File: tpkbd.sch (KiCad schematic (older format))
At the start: 21 parts, among them CON1 AVR-ISP-6, J1 CONN_01X02, J2 CONN_01X01, J3 USB_OTG, J4 CONN_02X20, J5 CONN_01X04, J6 GS2, J7 0, U1 ATMEGA8515-16AU, U2 AP111733, Y1 Crystal_GND24

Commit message: cleanup
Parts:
- removed CON1: AVR-ISP-6, Pin_Headers:Pin_Header_Straight_2x03, symbol AVR-ISP-6
- added D1: LED, KX14:PLCC4, symbol LED_Dual_AACC
- added J?: CONN_02X10, symbol CONN_02X10
- added R6, R7, R8: R, Resistors_SMD:R_0603_HandSoldering, symbol R
- C1, C2: footprint Capacitors_SMD:C_0805_HandSoldering -> Capacitors_SMD:C_0603_HandSoldering
- C3: footprint Capacitors_SMD:C_0402 -> Capacitors_SMD:C_0603_HandSoldering
- J2: footprint Pin_Headers:Pin_Header_Straight_1x01 -> KX14:Pins1x1
- J4: value CONN_02X20 -> CONN_02X21; symbol CONN_02X20 -> CONN_02X21
- R1, R2, R3, R4, R5: footprint Resistors_SMD:R_0805_HandSoldering -> Resistors_SMD:R_0603_HandSoldering
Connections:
- net +3V3: now also J?.2 (P2), R6.1; no longer J5.1 (P1)
- net +5V: now also J5.1 (P1)
- net B5: now also J?.4 (P4)
- net B6: now also J?.6 (P6)
- net B7: now also J?.8 (P8)
- net GND: now also J4.41 (P41), J?.12 (P12), R8.2
- net RST: now also J?.10 (P10)
- net kb_id0: now also R7.1; no longer U1.10 ((XCK)PD4)
- net at R3.2: now also U1.10 ((XCK)PD4); no longer U1.9 ((INT1)PD3)
- new net: D1.2 (A2), R6.2
- new net: D1.3 (K1), R8.1
- new net led: D1.1 (A1), D1.4 (K2), R7.2, U1.9 ((INT1)PD3)
- no-connect marks 4 -> 19
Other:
- moved on the sheet: J7, R3

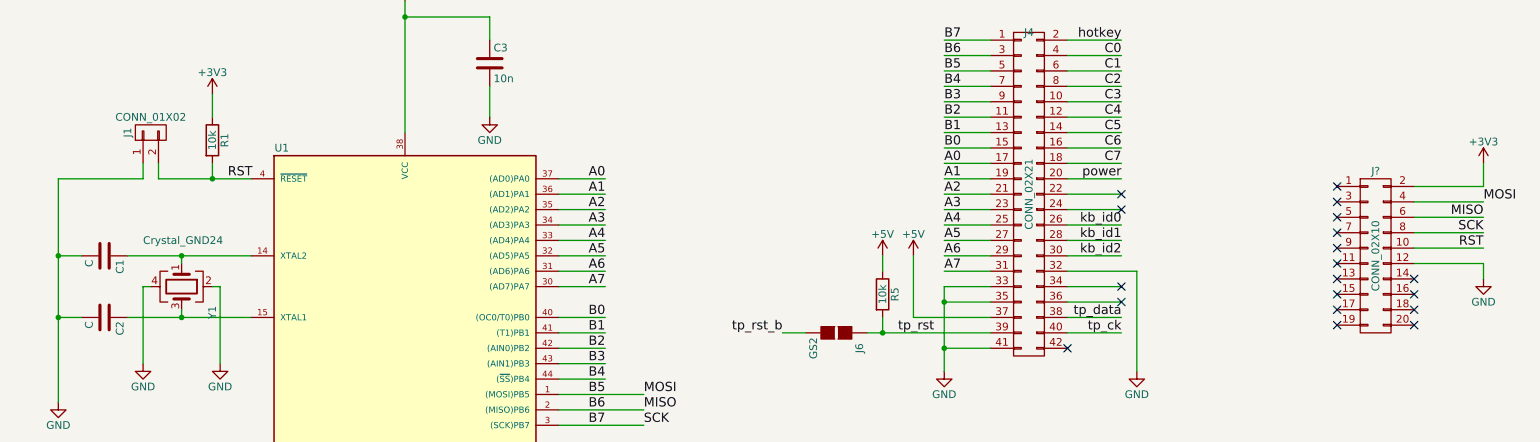
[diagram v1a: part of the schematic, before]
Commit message: cleanup2
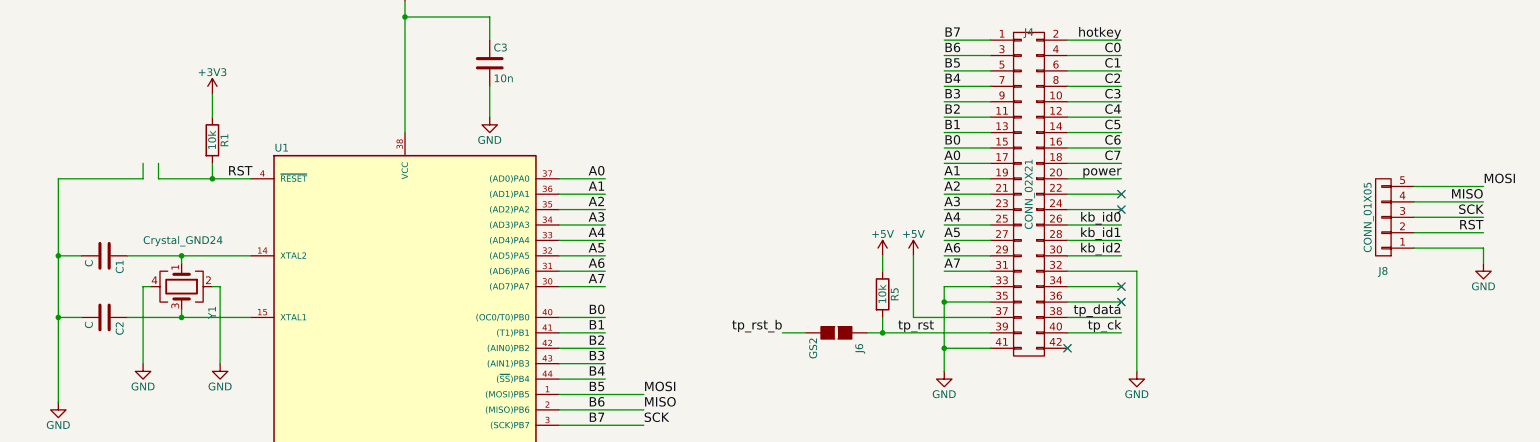
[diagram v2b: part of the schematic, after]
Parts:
- removed J1: CONN_01X02, Buttons_Switches_SMD:SW_SPST_FSMSM, symbol CONN_01X02
- removed J?: CONN_02X10, symbol CONN_02X10
- added J8: CONN_01X05, KX14:Pins_1x5, symbol CONN_01X05
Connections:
- net B5: now also J8.5 (P5)
- net B6: now also J8.4 (P4)
- net B7: now also J8.3 (P3)
- net GND: now also J8.1 (P1)
- net RST: now also J8.2 (P2)
- no-connect marks 19 -> 5
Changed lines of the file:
@@
-$EndComp
-$Comp
-L CONN_01X02 J1
-U 1 1 59BAB43F
-P 1900 2300
-F 0 "J1" H 1900 2450 50  0000 C CNN
-F 1 "CONN_01X02" V 2000 2300 50  0000 C CNN
-F 2 "Buttons_Switches_SMD:SW_SPST_FSMSM" H 1900 2300 50  0001 C CNN
-F 3 "" H 1900 2300 50  0001 C CNN
-	1    1900 2300
-	0    -1   -1   0
 $EndComp
 $Comp
@@
 Text Label 2400 2600 0    60   ~ 0
 RST
-Text Label 10550 3050 2    60   ~ 0
+Text Label 10550 2950 2    60   ~ 0
 RST
 Text Label 7050 2500 0    60   ~ 0
@@
 Connection ~ 6150 5000
 Wire Wire Line
-	10550 3050 10100 3050
+	10550 2950 10100 2950
+Wire Wire Line
+	10550 2750 10100 2750
 Wire Wire Line
 	10550 2850 10100 2850
 Wire Wire Line
-	10550 2950 10100 2950
-Wire Wire Line
 	10100 2650 10550 2650
 Wire Wire Line
-	10100 2750 10550 2750
-Wire Wire Line
-	10100 3150 10550 3150
+	10100 3050 10550 3050
 Wire Wire Line
 	7350 2500 7050 2500
@@
 Wire Wire Line
 	4550 5100 4900 5100
+Text Label 10550 2750 2    60   ~ 0
+MISO
 Text Label 10550 2850 2    60   ~ 0
-MISO
-Text Label 10550 2950 2    60   ~ 0
 SCK
-Text Label 10550 2750 0    60   ~ 0
+Text Label 10550 2650 0    60   ~ 0
 MOSI
 $Comp
 L GND #PWR014
 U 1 1 59BAD155
-P 10550 3250
-F 0 "#PWR014" H 10550 3000 50  0001 C CNN
-F 1 "GND" H 10550 3100 50  0000 C CNN
-F 2 "" H 10550 3250 50  0001 C CNN
-F 3 "" H 10550 3250 50  0001 C CNN
-	1    10550 3250
-	1    0    0    -1
-$EndComp
-Wire Wire Line
-	10550 3150 10550 3250
+P 10550 3150
+F 0 "#PWR014" H 10550 2900 50  0001 C CNN
+F 1 "GND" H 10550 3000 50  0000 C CNN
+F 2 "" H 10550 3150 50  0001 C CNN
+F 3 "" H 10550 3150 50  0001 C CNN
+	1    10550 3150
+	1    0    0    -1
+$EndComp
+Wire Wire Line
+	10550 3050 10550 3150
 Text Label 5100 4100 0    60   ~ 0
 MISO
@@
 	6900 4850 6900 5000
 Connection ~ 6900 5000
-$Comp
-L +3V3 #PWR017
-U 1 1 59BADCC0
-P 10550 2500
-F 0 "#PWR017" H 10550 2350 50  0001 C CNN
-F 1 "+3V3" H 10550 2640 50  0000 C CNN
-F 2 "" H 10550 2500 50  0001 C CNN
-F 3 "" H 10550 2500 50  0001 C CNN
-	1    10550 2500
-	1    0    0    -1
-$EndComp
-Wire Wire Line
-	10550 2650 10550 2500
 Wire Wire Line
 	4100 2200 4100 2000
@@
 	5350 5400 5350 5100
 $Comp
-L GND #PWR018
+L GND #PWR017
 U 1 1 59BAE839
 P 5450 6100
-F 0 "#PWR018" H 5450 5850 50  0001 C CNN
+F 0 "#PWR017" H 5450 5850 50  0001 C CNN
 F 1 "GND" H 5450 5950 50  0000 C CNN
 F 2 "" H 5450 6100 50  0001 C CNN
@@
 	5050 5100 5150 5100
 $Comp
-L PWR_FLAG #FLG019
+L PWR_FLAG #FLG018
 U 1 1 59BAEACE
 P 9100 5450
-F 0 "#FLG019" H 9100 5525 50  0001 C CNN
+F 0 "#FLG018" H 9100 5525 50  0001 C CNN
 F 1 "PWR_FLAG" H 9100 5600 50  0000 C CNN
 F 2 "" H 9100 5450 50  0001 C CNN
@@
 Connection ~ 8500 5600
 $Comp
-L PWR_FLAG #FLG020
+L PWR_FLAG #FLG019
 U 1 1 59BAEC2F
 P 9450 4900
-F 0 "#FLG020" H 9450 4975 50  0001 C CNN
+F 0 "#FLG019" H 9450 4975 50  0001 C CNN
 F 1 "PWR_FLAG" H 9450 5050 50  0000 C CNN
 F 2 "" H 9450 4900 50  0001 C CNN
@@
 $EndComp
 $Comp
-L GND #PWR021
+L GND #PWR020
 U 1 1 59BAF57F
 P 1850 3800
-F 0 "#PWR021" H 1850 3550 50  0001 C CNN
+F 0 "#PWR020" H 1850 3550 50  0001 C CNN
 F 1 "GND" H 1850 3650 50  0000 C CNN
 F 2 "" H 1850 3800 50  0001 C CNN
@@
 	1850 3300 1900 3300
 $Comp
-L GND #PWR022
+L GND #PWR021
 U 1 1 59BAF671
 P 2350 3800
-F 0 "#PWR022" H 2350 3550 50  0001 C CNN
+F 0 "#PWR021" H 2350 3550 50  0001 C CNN
 F 1 "GND" H 2350 3650 50  0000 C CNN
 F 2 "" H 2350 3800 50  0001 C CNN
@@
 	750  6250 750  6350
 $Comp
-L GND #PWR023
+L GND #PWR022
 U 1 1 59BB2E4B
 P 1350 7350
-F 0 "#PWR023" H 1350 7100 50  0001 C CNN
+F 0 "#PWR022" H 1350 7100 50  0001 C CNN
 F 1 "GND" H 1350 7200 50  0000 C CNN
 F 2 "" H 1350 7350 50  0001 C CNN
@@
 	1350 6950 1350 7350
 $Comp
-L PWR_FLAG #FLG024
+L PWR_FLAG #FLG023
 U 1 1 59BB3276
 P 7050 5850
-F 0 "#FLG024" H 7050 5925 50  0001 C CNN
+F 0 "#FLG023" H 7050 5925 50  0001 C CNN
 F 1 "PWR_FLAG" H 7050 6000 50  0000 C CNN
 F 2 "" H 7050 5850 50  0001 C CNN
@@
 NoConn ~ 7850 3700
 $Comp
-L +3V3 #PWR025
+L +3V3 #PWR024
 U 1 1 59BBC4D0
 P 750 5800
-F 0 "#PWR025" H 750 5650 50  0001 C CNN
+F 0 "#PWR024" H 750 5650 50  0001 C CNN
 F 1 "+3V3" H 750 5940 50  0000 C CNN
 F 2 "" H 750 5800 50  0001 C CNN
@@
 $EndComp
 $Comp
-L +5V #PWR026
+L +5V #PWR025
 U 1 1 59BBCA91
 P 5050 4700
-F 0 "#PWR026" H 5050 4550 50  0001 C CNN
+F 0 "#PWR025" H 5050 4550 50  0001 C CNN
 F 1 "+5V" H 5050 4840 50  0000 C CNN
 F 2 "" H 5050 4700 50  0001 C CNN
@@
 $EndComp
 $Comp
-L CONN_02X10 J?
-U 1 1 59BBD507
-P 9850 3100
-F 0 "J?" H 9850 3650 50  0000 C CNN
-F 1 "CONN_02X10" V 9850 3100 50  0000 C CNN
-F 2 "" H 9850 1900 50  0001 C CNN
-F 3 "" H 9850 1900 50  0001 C CNN
-	1    9850 3100
-	1    0    0    -1
-$EndComp
-NoConn ~ 9600 2650
-NoConn ~ 9600 2750
-NoConn ~ 9600 2850
-NoConn ~ 9600 2950
-NoConn ~ 9600 3050
-NoConn ~ 9600 3150
-NoConn ~ 9600 3250
-NoConn ~ 9600 3350
-NoConn ~ 9600 3450
-NoConn ~ 9600 3550
-NoConn ~ 10100 3250
-NoConn ~ 10100 3350
-NoConn ~ 10100 3450
-NoConn ~ 10100 3550
+L CONN_01X05 J8
+U 1 1 59BBF4F8
+P 9900 2850
+F 0 "J8" H 9900 3200 50  0000 C CNN
+F 1 "CONN_01X05" V 10000 2850 50  0000 C CNN
+F 2 "KX14:Pins_1x5" H 9900 2850 50  0001 C CNN
+F 3 "" H 9900 2850 50  0001 C CNN
+	1    9900 2850
+	-1   0    0    1
+$EndComp
 $EndSCHEMATC
